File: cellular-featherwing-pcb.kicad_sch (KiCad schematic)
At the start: 65 parts, among them J1 SIM8060-6-0-14-00-A, J2 TSM-116-01-L-SV, J3 TSM-112-01-L-SV, J4 U.FL-R-SMT, U1 BG96, U2 TPS63020QDSJTQ1, U3 TXB0108DQSR, U4 MAX8868EUK30+T

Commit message: Files sent to jlpcb
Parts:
- U4: LCSC (none) -> C37970
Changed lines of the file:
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@@
+      (effects (font (size 1.27 1.27)) hide)
+    )
+    (property "LCSC" "C37970" (id 7) (at 240.03 33.02 0)
       (effects (font (size 1.27 1.27)) hide)
     )

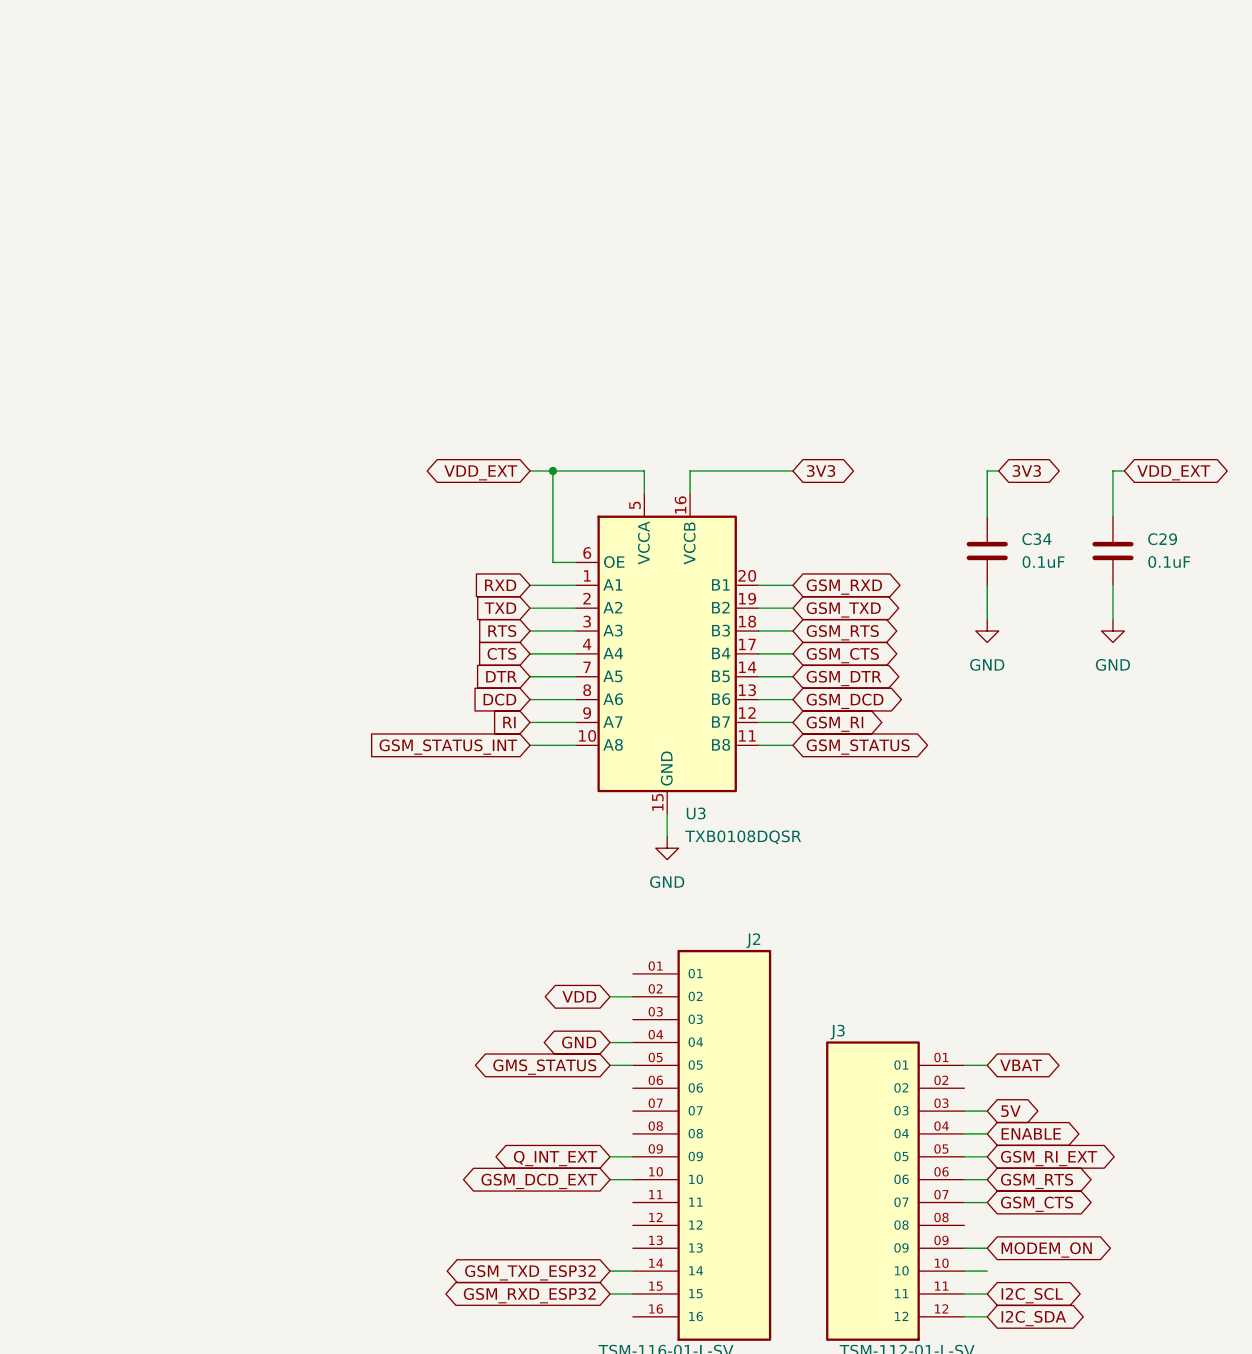
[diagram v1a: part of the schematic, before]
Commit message: Updates for jlpcb
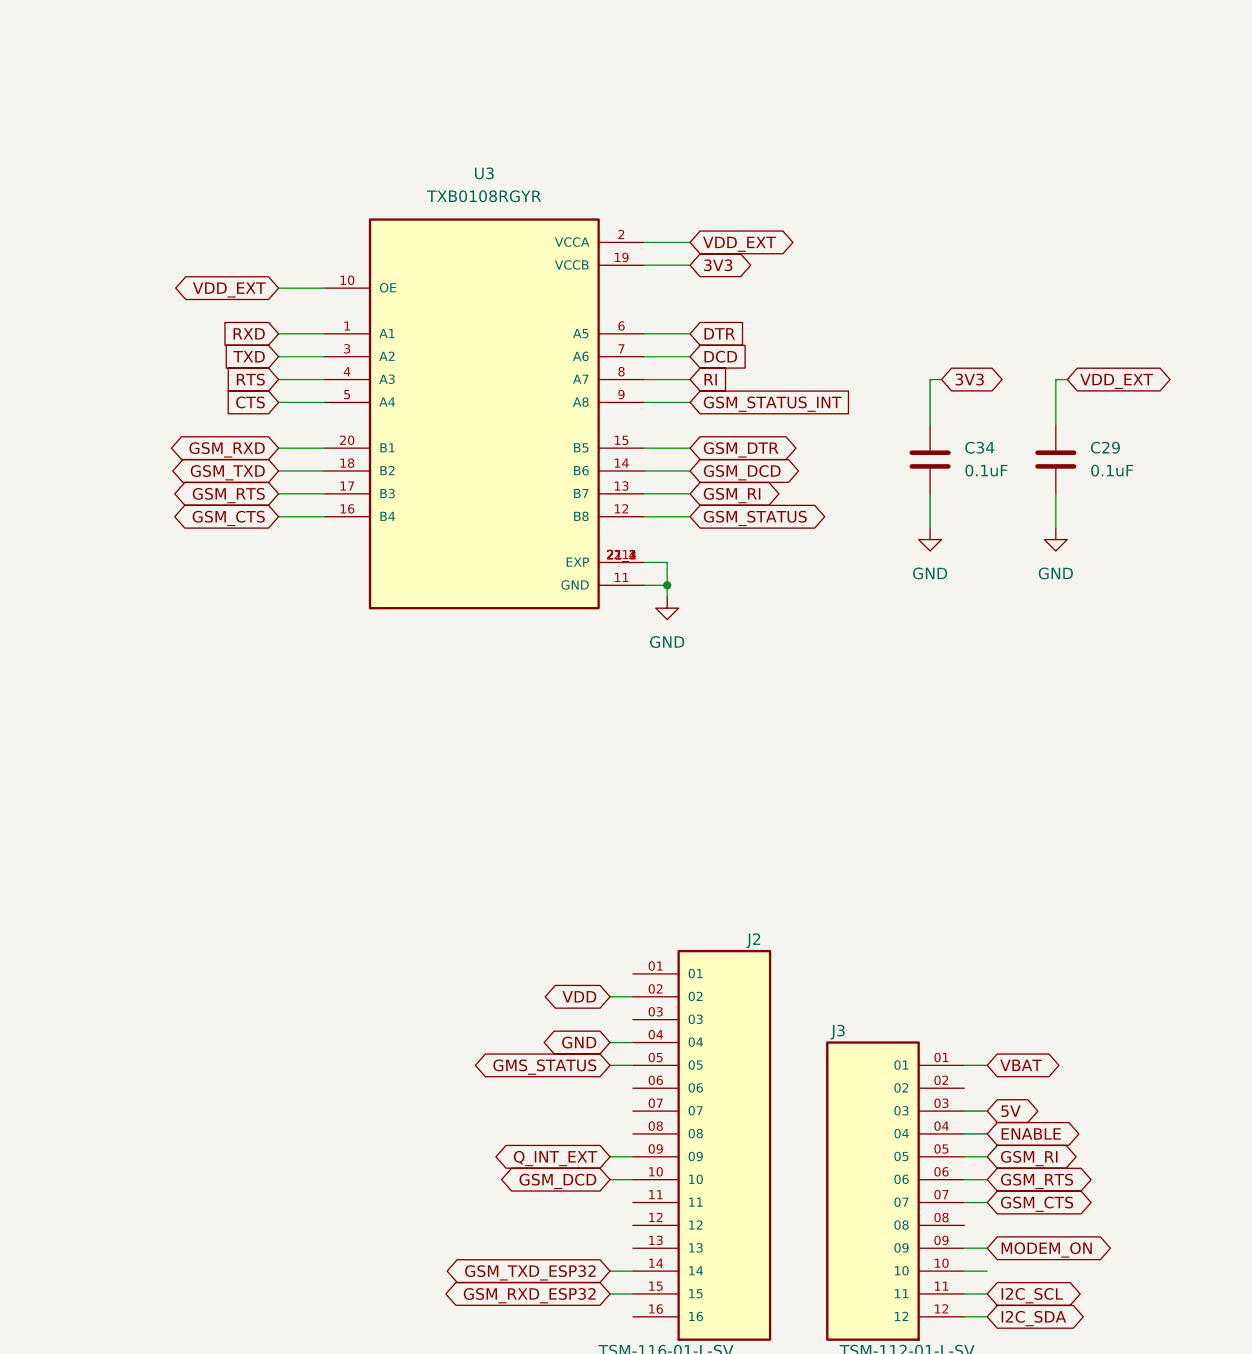
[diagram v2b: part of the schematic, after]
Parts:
- removed U3: TXB0108DQSR, Package_SON:USON-20_2x4mm_P0.4mm, symbol Logic_LevelTranslator:TXB0108DQSR
- added U3: TXB0108RGYR, IC_TXB0108RGYR, symbol TXB0108RGYR:TXB0108RGYR
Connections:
- net GSM_DCD_EXT is gone; now on net GSM_DCD: J2.10
- net GSM_RI_EXT is gone; now on net GSM_RI: J3.05
- net 3V3: now also U3.19 (VCCB)
- net CTS: now also U3.5 (A4)
- net DCD: now also U3.7 (A6)
- net DTR: now also U3.6 (A5)
- net GND: now also U3.11 (GND), U3.21 (EXP), U3.21_1 (EXP), U3.21_2 (EXP), U3.21_3 (EXP), U3.21_4 (EXP)
- net GSM_CTS: now also U3.16 (B4)
- net GSM_DCD: now also U3.14 (B6)
- net GSM_DTR: now also U3.15 (B5)
- net GSM_RI: now also U3.13 (B7)
- net GSM_RTS: now also U3.17 (B3)
- net GSM_RXD: now also U3.20 (B1)
- net GSM_STATUS: now also U3.12 (B8)
- net GSM_STATUS_INT: now also U3.9 (A8)
- net GSM_TXD: now also U3.18 (B2)
- net RI: now also U3.8 (A7)
- net RTS: now also U3.4 (A3)
- net RXD: now also U3.1 (A1)
- net TXD: now also U3.3 (A2)
- net VDD_EXT: now also U3.10 (OE), U3.2 (VCCA)
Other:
- moved on the sheet: C29, C34
